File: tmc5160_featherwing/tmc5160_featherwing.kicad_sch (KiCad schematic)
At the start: 0 parts

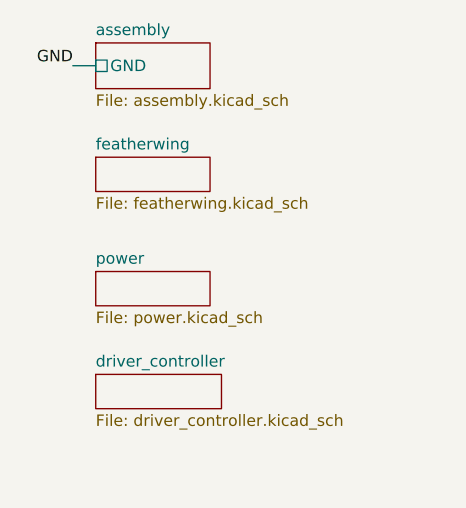
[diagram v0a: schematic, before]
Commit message: Add to power sheet
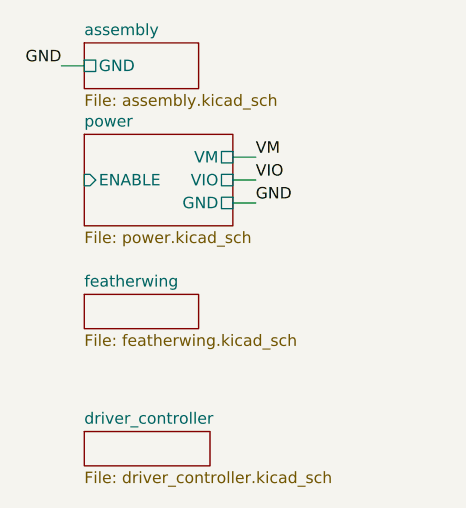
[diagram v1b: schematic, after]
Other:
- sheet power ports: added ENABLE, GND, VIO, VM; removed none
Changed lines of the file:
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@@
   (title_block
     (title "tmc5160_featherwing")
-    (date "2024-04-04")
+    (date "2024-04-05")
     (rev "1.0")
     (company "Howard Hughes Medical Institute")
   )
-  (wire (pts (xy 57.15 38.1) (xy 59.69 38.1))
+  (wire (pts (xy 77.47 48.26) (xy 74.93 48.26))
     (stroke (width 0) (type default))
   )
-  (label "GND" (at 57.15 38.1 180) (fields_autoplaced)
+  (wire (pts (xy 55.88 38.1) (xy 58.42 38.1))
+    (stroke (width 0) (type default))
+  )
+  (wire (pts (xy 77.47 53.34) (xy 74.93 53.34))
+    (stroke (width 0) (type default))
+  )
+  (wire (pts (xy 77.47 50.8) (xy 74.93 50.8))
+    (stroke (width 0) (type default))
+  )
+  (label "GND" (at 77.47 53.34 0) (fields_autoplaced)
+    (effects (font (size 1.27 1.27)) (justify left bottom))
+  )
+  (label "VIO" (at 77.47 50.8 0) (fields_autoplaced)
+    (effects (font (size 1.27 1.27)) (justify left bottom))
+  )
+  (label "GND" (at 55.88 38.1 180) (fields_autoplaced)
     (effects (font (size 1.27 1.27)) (justify right bottom))
   )
-  (sheet (at 59.69 72.39) (size 13.97 3.81) (fields_autoplaced)
+  (label "VM" (at 77.47 48.26 0) (fields_autoplaced)
+    (effects (font (size 1.27 1.27)) (justify left bottom))
+  )
+  (sheet (at 58.42 78.74) (size 13.97 3.81) (fields_autoplaced)
     (stroke (width 0.1524) (type solid))
     (fill (color 0 0 0 0.0000))
-    (property "Sheetname" "driver_controller" (at 59.69 71.6784 0)
+    (property "Sheetname" "driver_controller" (at 58.42 78.0284 0)
       (effects (font (size 1.27 1.27)) (justify left bottom))
     )
-    (property "Sheetfile" "driver_controller.kicad_sch" (at 59.69 76.7846 0)
+    (property "Sheetfile" "driver_controller.kicad_sch" (at 58.42 83.1346 0)
       (effects (font (size 1.27 1.27)) (justify left top))
     )
@@
     )
   )
-  (sheet (at 59.69 35.56) (size 12.7 5.08) (fields_autoplaced)
+  (sheet (at 58.42 35.56) (size 12.7 5.08) (fields_autoplaced)
     (stroke (width 0.1524) (type solid))
     (fill (color 0 0 0 0.0000))
-    (property "Sheetname" "assembly" (at 59.69 34.8484 0)
+    (property "Sheetname" "assembly" (at 58.42 34.8484 0)
       (effects (font (size 1.27 1.27)) (justify left bottom))
     )
-    (property "Sheetfile" "assembly.kicad_sch" (at 59.69 41.2246 0)
+    (property "Sheetfile" "assembly.kicad_sch" (at 58.42 41.2246 0)
       (effects (font (size 1.27 1.27)) (justify left top))
     )
-    (pin "GND" passive (at 59.69 38.1 180)
+    (pin "GND" passive (at 58.42 38.1 180)
       (effects (font (size 1.27 1.27)) (justify left))
     )
@@
     )
   )
-  (sheet (at 59.69 48.26) (size 12.7 3.81) (fields_autoplaced)
+  (sheet (at 58.42 63.5) (size 12.7 3.81) (fields_autoplaced)
     (stroke (width 0.1524) (type solid))
     (fill (color 0 0 0 0.0000))
-    (property "Sheetname" "featherwing" (at 59.69 47.5484 0)
+    (property "Sheetname" "featherwing" (at 58.42 62.7884 0)
       (effects (font (size 1.27 1.27)) (justify left bottom))
     )
-    (property "Sheetfile" "featherwing.kicad_sch" (at 59.69 52.6546 0)
+    (property "Sheetfile" "featherwing.kicad_sch" (at 58.42 67.8946 0)
       (effects (font (size 1.27 1.27)) (justify left top))
     )
@@
     )
   )
-  (sheet (at 59.69 60.96) (size 12.7 3.81) (fields_autoplaced)
+  (sheet (at 58.42 45.72) (size 16.51 10.16) (fields_autoplaced)
     (stroke (width 0.1524) (type solid))
     (fill (color 0 0 0 0.0000))
-    (property "Sheetname" "power" (at 59.69 60.2484 0)
+    (property "Sheetname" "power" (at 58.42 45.0084 0)
       (effects (font (size 1.27 1.27)) (justify left bottom))
     )
-    (property "Sheetfile" "power.kicad_sch" (at 59.69 65.3546 0)
+    (property "Sheetfile" "power.kicad_sch" (at 58.42 56.4646 0)
       (effects (font (size 1.27 1.27)) (justify left top))
     )
+    (pin "GND" passive (at 74.93 53.34 0)
+      (effects (font (size 1.27 1.27)) (justify right))
+    )
+    (pin "VM" passive (at 74.93 48.26 0)
+      (effects (font (size 1.27 1.27)) (justify right))
+    )
+    (pin "VIO" passive (at 74.93 50.8 0)
+      (effects (font (size 1.27 1.27)) (justify right))
+    )
+    (pin "ENABLE" input (at 58.42 50.8 180)
+      (effects (font (size 1.27 1.27)) (justify left))
+    )
     (instances
